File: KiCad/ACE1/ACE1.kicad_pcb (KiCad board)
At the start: 2 copper layers, 198.1 x 200.7 mm, 147 parts, among them IC1 78T, Q1 2N3904, Q2 2N2369, Q3 BC183, Q4 2N3904, X1 6.556MHz

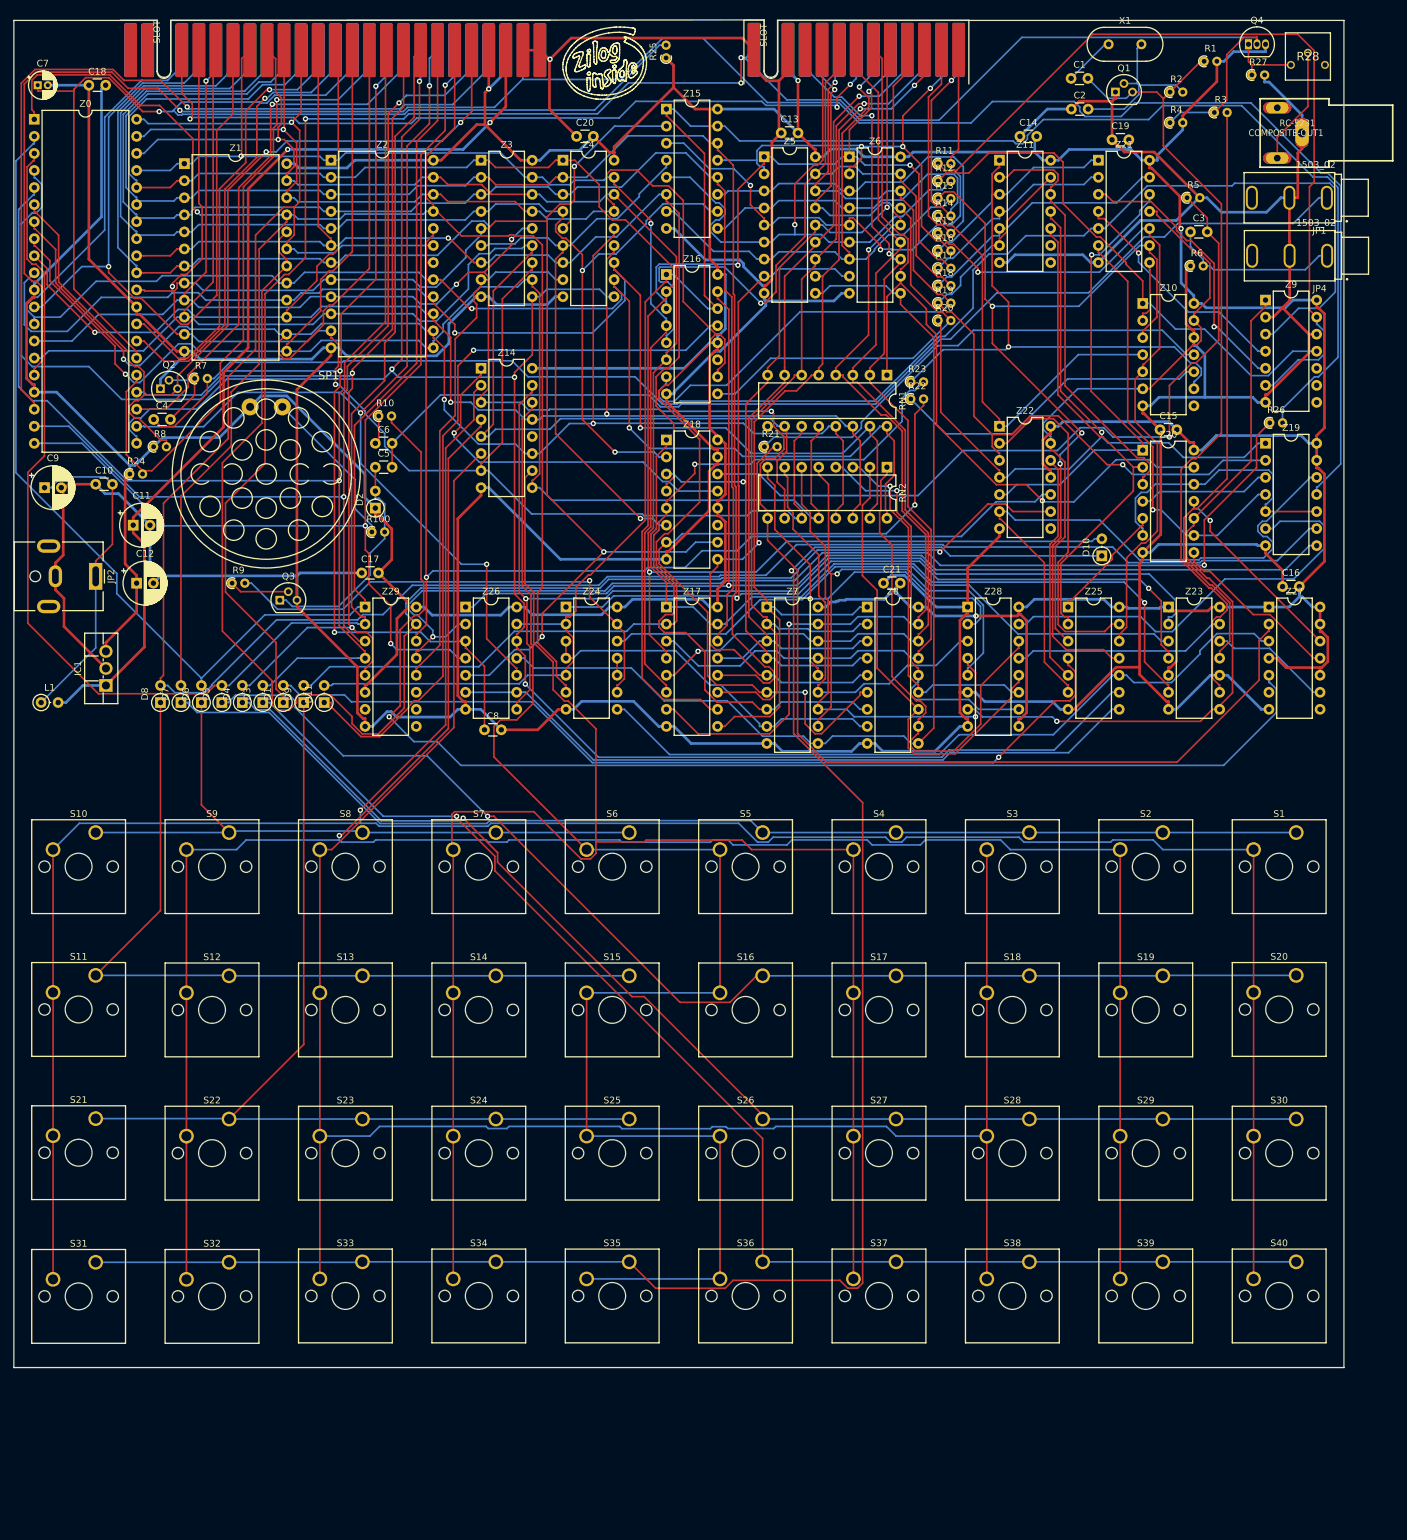
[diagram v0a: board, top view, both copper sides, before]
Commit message: Add space key. Re-jig PCB positions.
Signed-off-by: John Bradley <flypie@rocketmail.com>
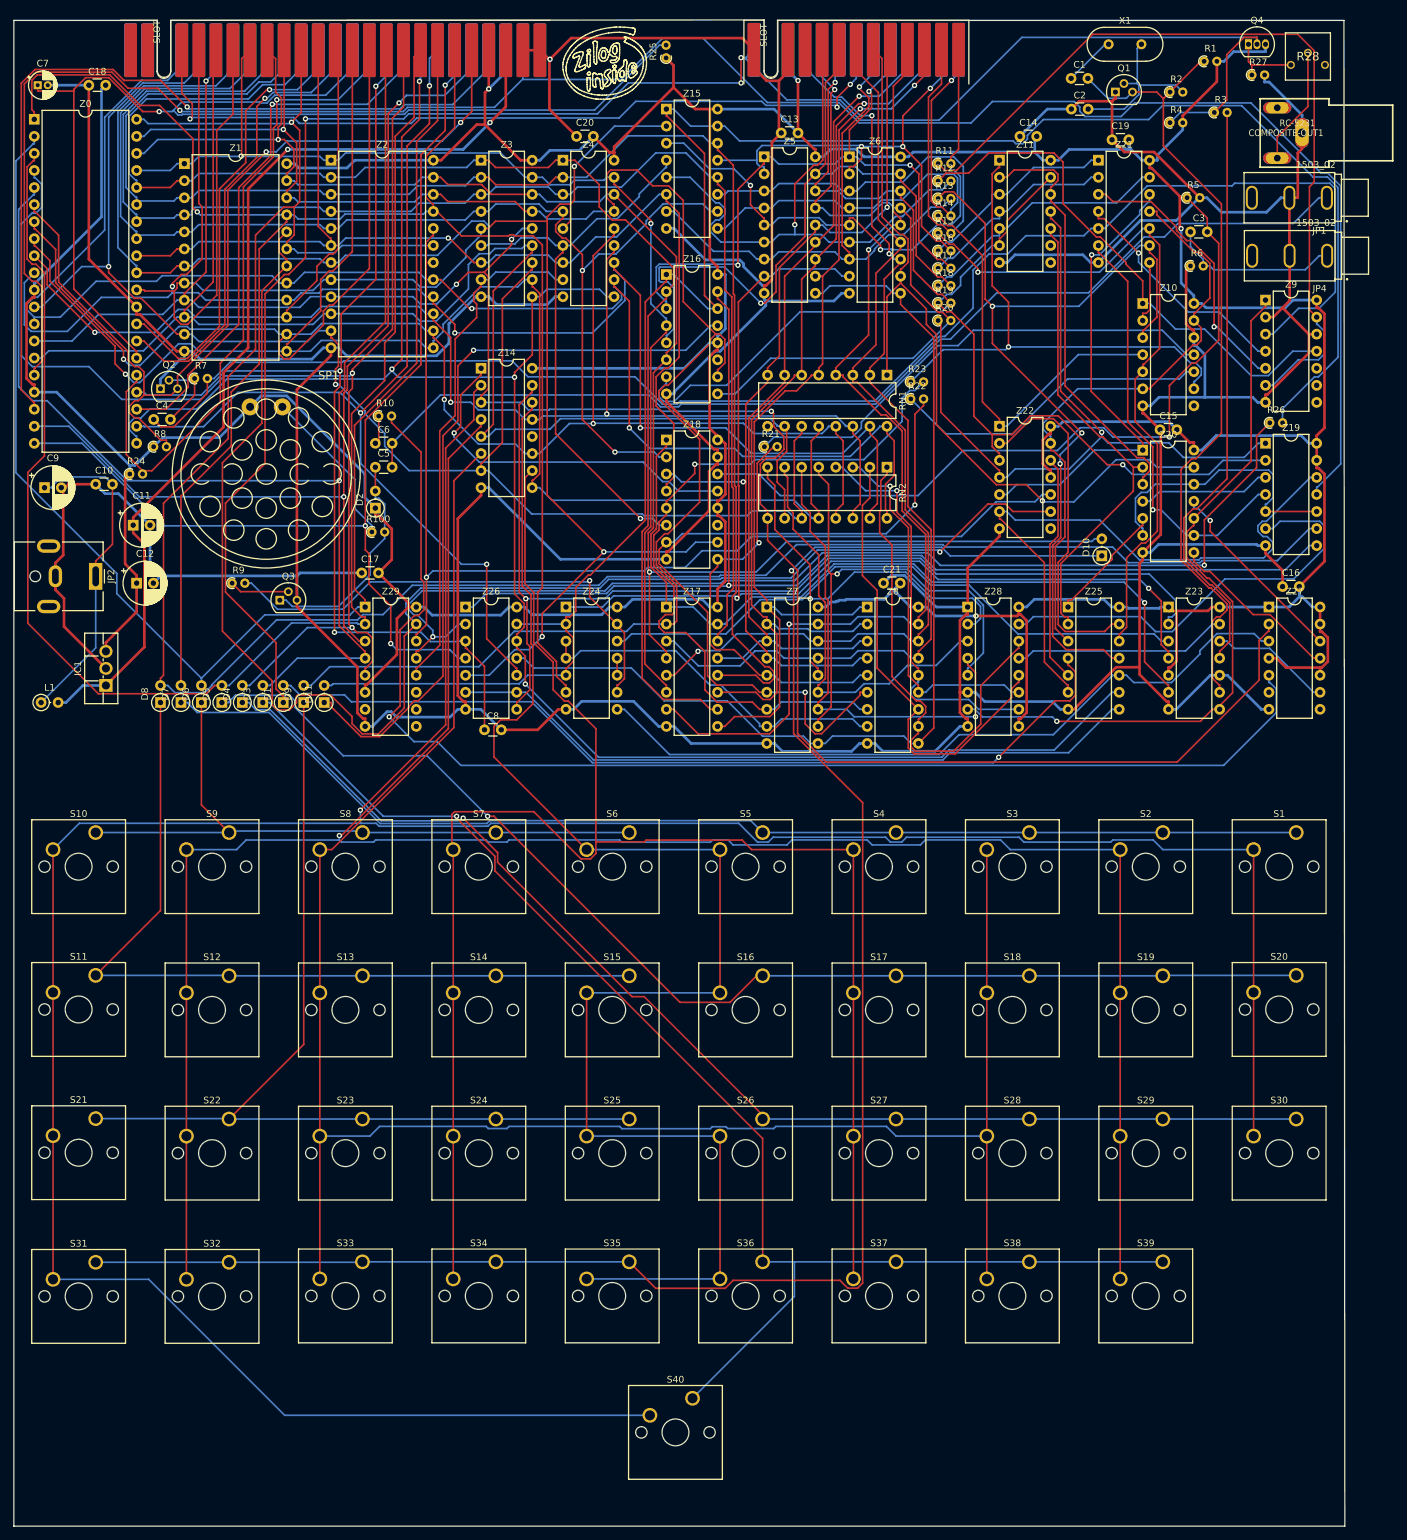
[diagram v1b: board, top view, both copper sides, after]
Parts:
- moved S40 92.2 mm to (177.8, 248.9)
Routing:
- net Net-(S1-Pad2): track 384.5 -> 460.5 mm
- net Net-(D3-Pad1): track 200.7 -> 207.4 mm
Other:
- board size 198.1 x 200.7 mm -> 198.2 x 224.4 mm

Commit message: ACE2NOKBV2MK2 update IC placement. Reverse Diode.
Signed-off-by: John Bradley <flypie@rocketmail.com>
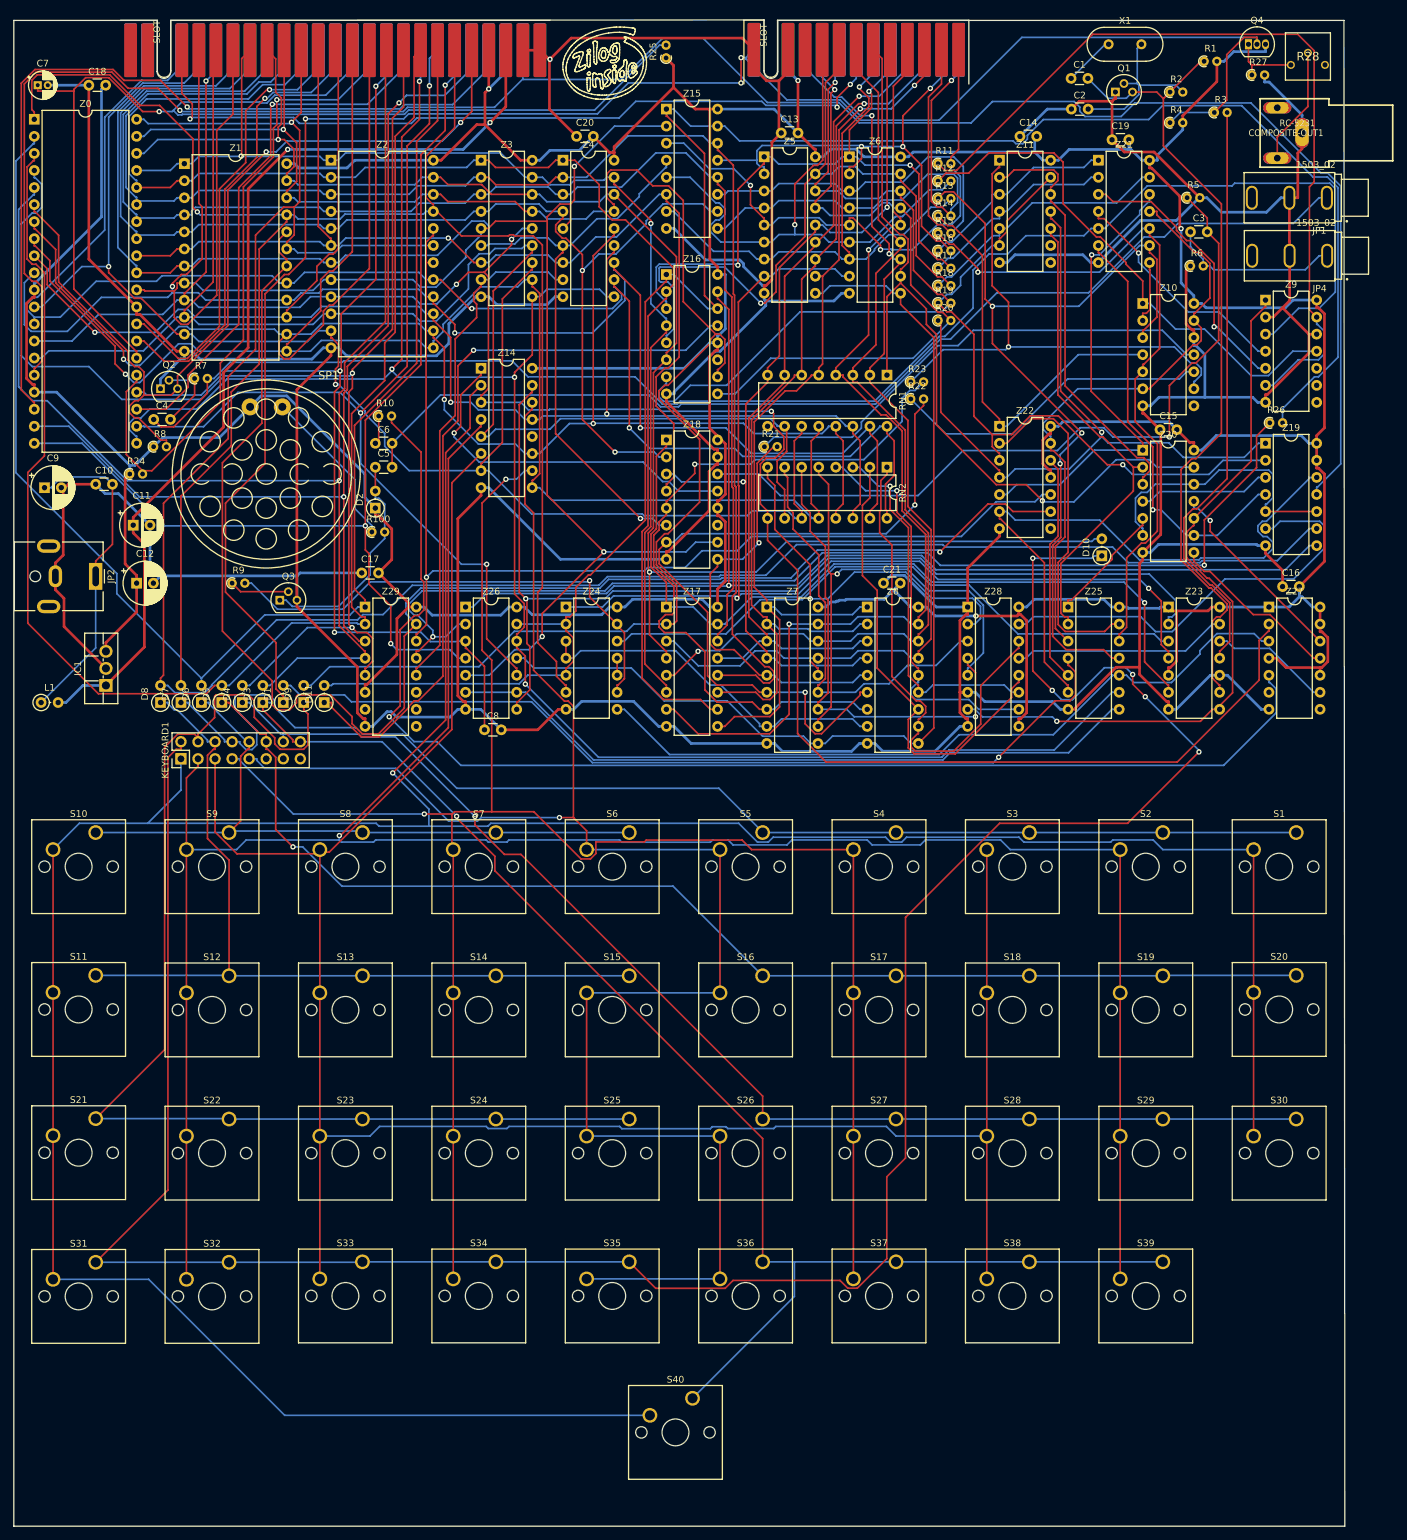
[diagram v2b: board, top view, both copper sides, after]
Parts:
- added KEYBOARD1: Conn_02x08_Odd_Even, Connector_PinHeader_2.54mm:PinHeader_2x08_P2.54mm_Vertical, F.Cu at (101.6, 153.7)
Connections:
- net Net-(D10-Pad1) renamed /ROW8
- net Net-(D3-Pad1) renamed /ROW15
- net Net-(D4-Pad1) renamed /ROW14
- net Net-(D5-Pad1) renamed /ROW13
- net Net-(D6-Pad1) renamed /ROW12
- net Net-(D7-Pad1) renamed /ROW11
- net Net-(D8-Pad1) renamed /ROW10
- net Net-(D9-Pad1) renamed /ROW9
- net Net-(S1-Pad2) renamed /COLA
- net Net-(S12-Pad2) renamed /COLB
- net Net-(S13-Pad2) renamed /COLC
- net Net-(S14-Pad2) renamed /COLD
- net Net-(S15-Pad2) renamed /COLE
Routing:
- net /ROW8: track 275.9 -> 373.3 mm, vias 1 -> 5
- net /COLE: track 220.9 -> 267.2 mm, vias 0 -> 1
- net /ROW9: track 146.1 -> 179.0 mm
- net /COLD: track 259.3 -> 291.2 mm, vias 0 -> 2
- net /COLC: track 299.2 -> 327.2 mm
- net /ROW11: track 174.6 -> 190.8 mm
- net /COLB: track 341.9 -> 356.2 mm
- net /COLA: track 460.5 -> 472.9 mm
- net /ROW13: track 181.8 -> 185.5 mm
- net /ROW12: track 100.7 -> 104.2 mm
- net /ROW10: track 124.1 -> 127.1 mm
- net /ROW14: track 184.3 -> 186.6 mm
- net /ROW15: track 207.4 -> 209.3 mm
